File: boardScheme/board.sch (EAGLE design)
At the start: 24 parts, among them IC1 MEGA32-P, Q1 BC547, Q10 BC547, Q11 BC547, Q12 BC547, Q13 BC547, Q14 BC547, Q2 BC547, Q3 BC547, Q4 BC547, Q5 BC547, Q6 BC547, Q7 BC547, Q8 BC547, Q9 BC547

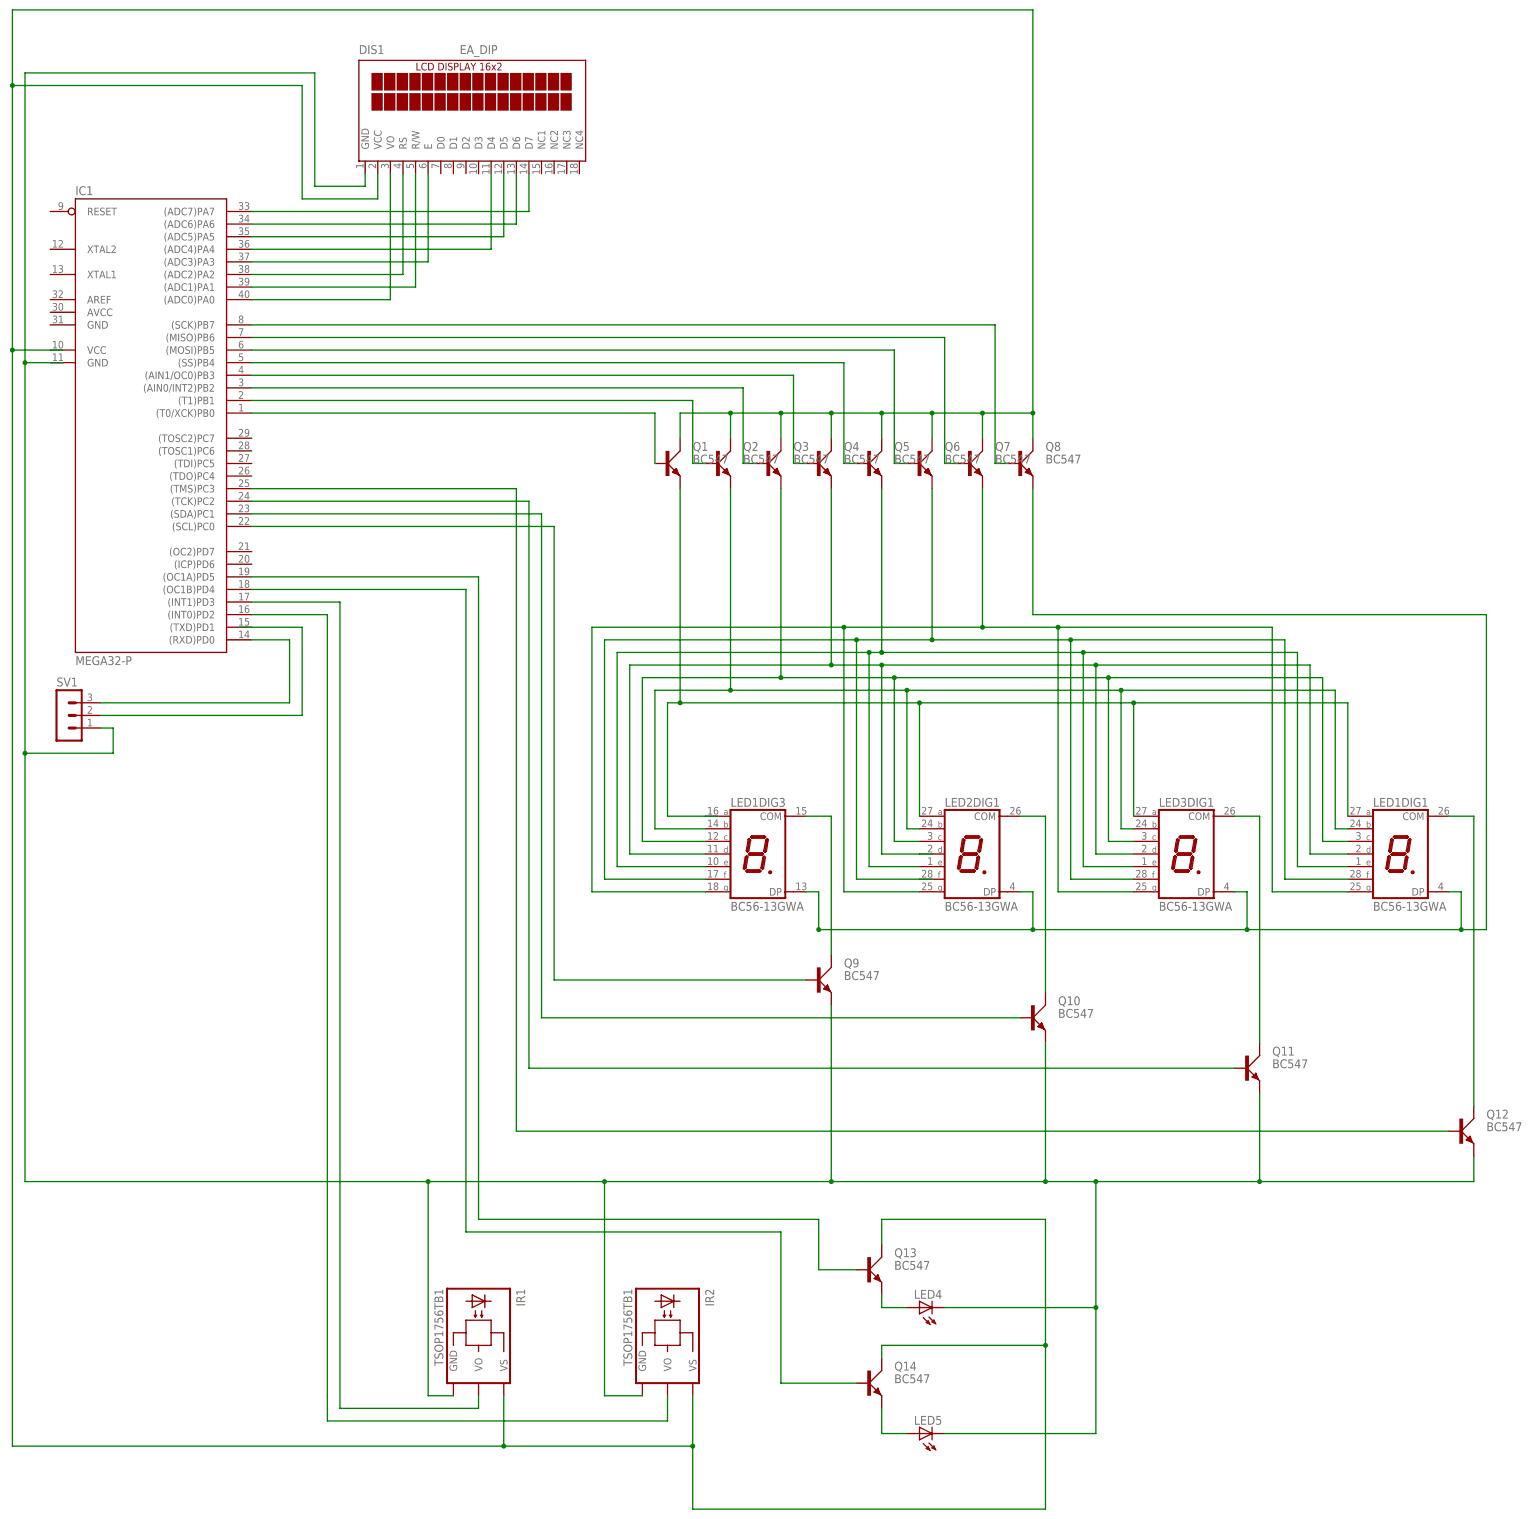
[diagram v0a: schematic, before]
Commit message: Changed board scheme.
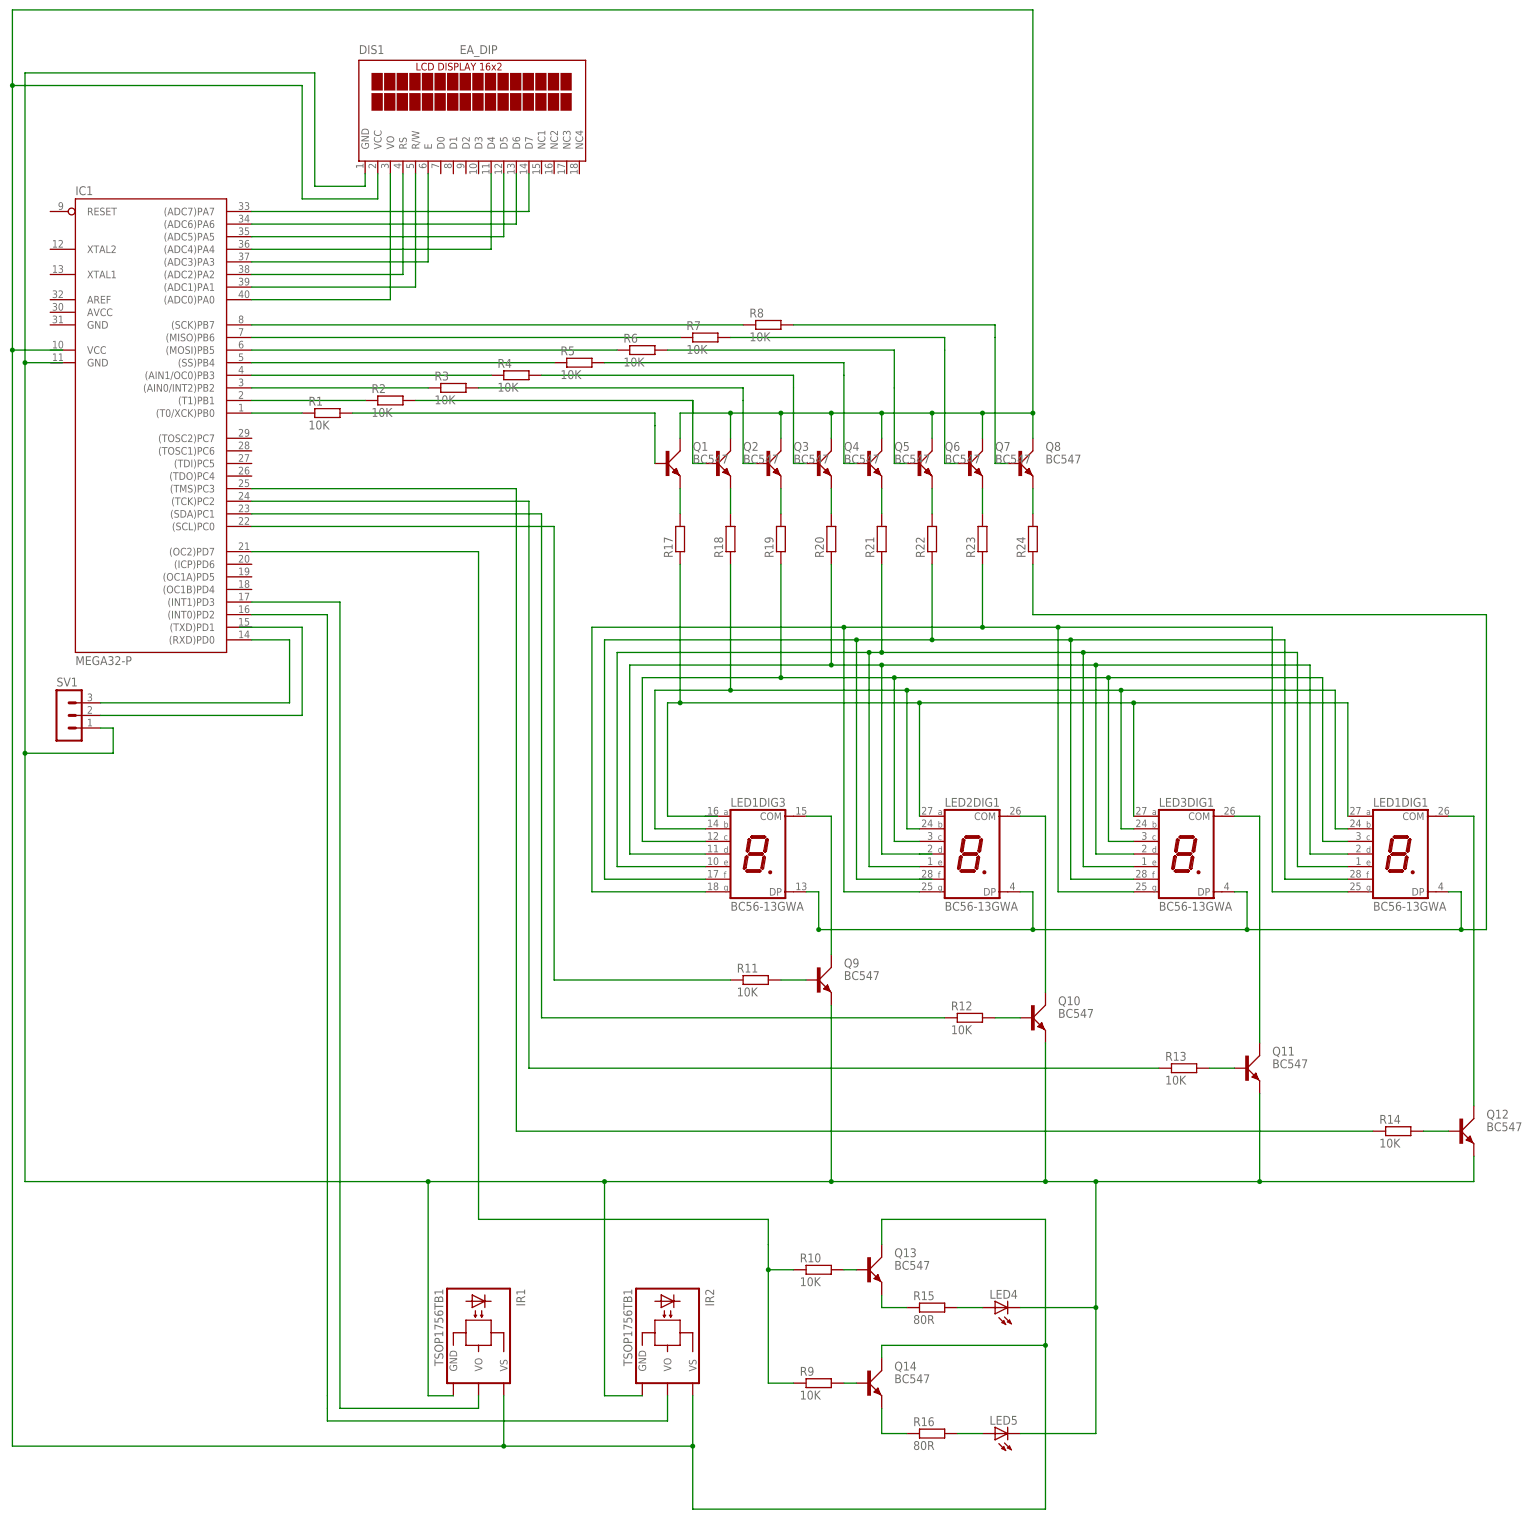
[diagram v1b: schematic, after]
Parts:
- added R1, R10, R11, R12, R13, R14, R2, R3, R4, R5, R6, R7, R8, R9: 10K, eagle-ltspice:R0204/7
- added R15, R16: 80R, eagle-ltspice:R0204/7
- added R17, R18, R19, R20, R21, R22, R23, R24: (no value), eagle-ltspice:R0204/7
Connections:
- new net N$23: Q2.B
- new net N$25: Q1.B, R1.2
- new net N$30: IC1.(AIN0/INT2)PB2, R3.1
- new net N$31: IC1.(AIN1/OC0)PB3, R4.1
- new net N$32: IC1.(SS)PB4, R5.1
- new net N$33: IC1.(MOSI)PB5, R6.1
- new net N$49: IC1.(MISO)PB6, R7.1
- new net N$50: IC1.(SCK)PB7, R8.1
- new net N$51: Q14.B, R9.2
- new net N$53: Q9.B, R11.2
- new net N$54: Q11.B, R13.2
- new net N$55: Q10.B, R12.2
- new net N$56: Q12.B, R14.2
- new net N$57: LED4.A, R15.2
- new net N$58: LED5.A, R16.2
- new net N$59: Q1.E, R17.2
- new net N$60: Q2.E, R18.2
- new net N$61: Q3.E, R19.2
- new net N$62: Q4.E, R20.2
- new net N$63: Q5.E, R21.2
- new net N$64: Q6.E, R22.2
- new net N$65: Q7.E, R23.2
- new net N$66: Q8.E, R24.2
- net N$11: now also R1.1; no longer Q1.B
- net N$13: now also R2.2
- net N$14: now also R2.1; no longer Q2.B
- net N$15: now also R3.2; no longer IC1.(AIN0/INT2)PB2
- net N$16: now also R4.2; no longer IC1.(AIN1/OC0)PB3
- net N$17: now also R5.2; no longer IC1.(SS)PB4
- net N$18: now also R6.2; no longer IC1.(MOSI)PB5
- net N$19: now also R7.2; no longer IC1.(MISO)PB6
- net N$20: now also R8.2; no longer IC1.(SCK)PB7
- net N$21: now also R17.1; no longer Q1.E
- net N$22: now also R20.1; no longer Q4.E
- net N$24: now also R18.1; no longer Q2.E
- net N$26: now also R19.1; no longer Q3.E
- net N$27: now also R23.1; no longer Q7.E
- net N$28: now also R21.1; no longer Q5.E
- net N$29: now also R11.1; no longer Q9.B
- net N$3: now also Q13.B, R10.2; no longer IC1.(OC1B)PD4, Q14.B
- net N$34: now also R12.1; no longer Q10.B
- net N$35: now also R24.1; no longer Q8.E
- net N$40: now also R13.1; no longer Q11.B
- net N$41: now also R14.1; no longer Q12.B
- net N$42: now also IC1.(OC2)PD7, R10.1, R9.1; no longer IC1.(OC1A)PD5, Q13.B
- net N$43: now also R15.1; no longer LED4.A
- net N$45: now also R16.1; no longer LED5.A
- net N$48: now also R22.1; no longer Q6.E
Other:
- moved on the sheet: LED4, LED5
